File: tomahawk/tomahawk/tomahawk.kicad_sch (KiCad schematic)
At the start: 79 parts, among them SW1 SW_Push, SW10 SW_Push, SW11 SW_Push, SW12 SW_Push, SW13 SW_Push, SW14 SW_Push, SW15 SW_Push, SW16 SW_Push, SW17 SW_Push, SW18 SW_Push, SW19 SW_Push, SW2 SW_Push, SW20 SW_Push, SW21 SW_Push, SW22 SW_Push, SW23 SW_Push, SW24 SW_Push, SW25 SW_Push, SW26 SW_Push, SW27 SW_Push, SW28 SW_Push, SW29 SW_Push, SW3 SW_Push, SW30 SW_Push, SW31 SW_Push, SW32 SW_Push, SW33 SW_Push, SW34 SW_Push, SW35 SW_Push, SW36 SW_Push, SW37 SW_Push, SW38 SW_Push, SW39 SW_Push, SW4 SW_Push, SW5 SW_Push, SW6 SW_Push, SW7 SW_Push, SW8 SW_Push, SW9 SW_Push

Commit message: updated footprints and pcb
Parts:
- SW1, SW10, SW11, SW12, SW13, SW14, SW15, SW16, SW17, SW18, SW19, SW2, SW20, SW21, SW22, SW23, SW24, SW25, SW26, SW27, SW28, SW29, SW3, SW30, SW31, SW32, SW33, SW34, SW35, SW36, SW37, SW38, SW39, SW4, SW5, SW6, SW7, SW8, SW9: footprint Keyswitches:Kailh_socket_PG1350 -> Foostan:keyswitch_choc12_hotswap_1u
- U1: footprint ProMicro_RP2040:pro_micro_rp2040 -> ProMicro RP2040:pro_micro_rp2040
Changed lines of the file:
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@@
 			)
 		)
-		(property "Footprint" "Keyswitches:Kailh_socket_PG1350"
+		(property "Footprint" "Foostan:keyswitch_choc12_hotswap_1u"
 			(at 43.18 90.17 0)
 			(effects
@@
 			)
 		)
-		(property "Footprint" "Keyswitches:Kailh_socket_PG1350"
+		(property "Footprint" "Foostan:keyswitch_choc12_hotswap_1u"
 			(at 43.18 33.02 0)
 			(effects
@@
 			)
 		)
-		(property "Footprint" "Keyswitches:Kailh_socket_PG1350"
+		(property "Footprint" "Foostan:keyswitch_choc12_hotswap_1u"
 			(at 119.38 90.17 0)
 			(effects
@@
 			)
 		)
-		(property "Footprint" "Keyswitches:Kailh_socket_PG1350"
+		(property "Footprint" "Foostan:keyswitch_choc12_hotswap_1u"
 			(at 138.43 33.02 0)
 			(effects
@@
 			)
 		)
-		(property "Footprint" "Keyswitches:Kailh_socket_PG1350"
+		(property "Footprint" "Foostan:keyswitch_choc12_hotswap_1u"
 			(at 119.38 147.32 0)
 			(effects
@@
 			)
 		)
-		(property "Footprint" "Keyswitches:Kailh_socket_PG1350"
+		(property "Footprint" "Foostan:keyswitch_choc12_hotswap_1u"
 			(at 43.18 52.07 0)
 			(effects
@@
 			)
 		)
-		(property "Footprint" "Keyswitches:Kailh_socket_PG1350"
+		(property "Footprint" "Foostan:keyswitch_choc12_hotswap_1u"
 			(at 81.28 147.32 0)
 			(effects
@@
 			)
 		)
-		(property "Footprint" "Keyswitches:Kailh_socket_PG1350"
+		(property "Footprint" "Foostan:keyswitch_choc12_hotswap_1u"
 			(at 81.28 71.12 0)
 			(effects
@@
 			)
 		)
-		(property "Footprint" "ProMicro_RP2040:pro_micro_rp2040"
+		(property "Footprint" "ProMicro RP2040:pro_micro_rp2040"
 			(at 198.12 31.75 0)
 			(effects
@@
 			)
 		)
-		(property "Footprint" "Keyswitches:Kailh_socket_PG1350"
+		(property "Footprint" "Foostan:keyswitch_choc12_hotswap_1u"
 			(at 100.33 128.27 0)
 			(effects
@@
 			)
 		)
-		(property "Footprint" "Keyswitches:Kailh_socket_PG1350"
+		(property "Footprint" "Foostan:keyswitch_choc12_hotswap_1u"
 			(at 138.43 109.22 0)
 			(effects
@@
 			)
 		)
-		(property "Footprint" "Keyswitches:Kailh_socket_PG1350"
+		(property "Footprint" "Foostan:keyswitch_choc12_hotswap_1u"
 			(at 100.33 71.12 0)
 			(effects
@@
 			)
 		)
-		(property "Footprint" "Keyswitches:Kailh_socket_PG1350"
+		(property "Footprint" "Foostan:keyswitch_choc12_hotswap_1u"
 			(at 138.43 90.17 0)
 			(effects
@@
 			)
 		)
-		(property "Footprint" "Keyswitches:Kailh_socket_PG1350"
+		(property "Footprint" "Foostan:keyswitch_choc12_hotswap_1u"
 			(at 62.23 52.07 0)
 			(effects
@@
 			)
 		)
-		(property "Footprint" "Keyswitches:Kailh_socket_PG1350"
+		(property "Footprint" "Foostan:keyswitch_choc12_hotswap_1u"
 			(at 62.23 109.22 0)
 			(effects
@@
 			)
 		)
-		(property "Footprint" "Keyswitches:Kailh_socket_PG1350"
+		(property "Footprint" "Foostan:keyswitch_choc12_hotswap_1u"
 			(at 43.18 71.12 0)
 			(effects
@@
 			)
 		)
-		(property "Footprint" "Keyswitches:Kailh_socket_PG1350"
+		(property "Footprint" "Foostan:keyswitch_choc12_hotswap_1u"
 			(at 100.33 90.17 0)
 			(effects
@@
 			)
 		)
-		(property "Footprint" "Keyswitches:Kailh_socket_PG1350"
+		(property "Footprint" "Foostan:keyswitch_choc12_hotswap_1u"
 			(at 119.38 71.12 0)
 			(effects
@@
 			)
 		)
-		(property "Footprint" "Keyswitches:Kailh_socket_PG1350"
+		(property "Footprint" "Foostan:keyswitch_choc12_hotswap_1u"
 			(at 119.38 52.07 0)
 			(effects
@@
 			)
 		)
-		(property "Footprint" "Keyswitches:Kailh_socket_PG1350"
+		(property "Footprint" "Foostan:keyswitch_choc12_hotswap_1u"
 			(at 119.38 33.02 0)
 			(effects
@@
 			)
 		)
-		(property "Footprint" "Keyswitches:Kailh_socket_PG1350"
+		(property "Footprint" "Foostan:keyswitch_choc12_hotswap_1u"
 			(at 81.28 33.02 0)
 			(effects
@@
 			)
 		)
-		(property "Footprint" "Keyswitches:Kailh_socket_PG1350"
+		(property "Footprint" "Foostan:keyswitch_choc12_hotswap_1u"
 			(at 100.33 166.37 0)
 			(effects
@@
 			)
 		)
-		(property "Footprint" "Keyswitches:Kailh_socket_PG1350"
+		(property "Footprint" "Foostan:keyswitch_choc12_hotswap_1u"
 			(at 138.43 52.07 0)
 			(effects
@@
 			)
 		)
-		(property "Footprint" "Keyswitches:Kailh_socket_PG1350"
+		(property "Footprint" "Foostan:keyswitch_choc12_hotswap_1u"
 			(at 100.33 52.07 0)
 			(effects
@@
 			)
 		)
-		(property "Footprint" "Keyswitches:Kailh_socket_PG1350"
+		(property "Footprint" "Foostan:keyswitch_choc12_hotswap_1u"
 			(at 81.28 128.27 0)
 			(effects
@@
 			)
 		)
-		(property "Footprint" "Keyswitches:Kailh_socket_PG1350"
+		(property "Footprint" "Foostan:keyswitch_choc12_hotswap_1u"
 			(at 62.23 71.12 0)
 			(effects
@@
 			)
 		)
-		(property "Footprint" "Keyswitches:Kailh_socket_PG1350"
+		(property "Footprint" "Foostan:keyswitch_choc12_hotswap_1u"
 			(at 81.28 166.37 0)
 			(effects
@@
 			)
 		)
-		(property "Footprint" "Keyswitches:Kailh_socket_PG1350"
+		(property "Footprint" "Foostan:keyswitch_choc12_hotswap_1u"
 			(at 100.33 109.22 0)
 			(effects
@@
 			)
 		)
-		(property "Footprint" "Keyswitches:Kailh_socket_PG1350"
+		(property "Footprint" "Foostan:keyswitch_choc12_hotswap_1u"
 			(at 81.28 109.22 0)
 			(effects
@@
 			)
 		)
-		(property "Footprint" "Keyswitches:Kailh_socket_PG1350"
+		(property "Footprint" "Foostan:keyswitch_choc12_hotswap_1u"
 			(at 119.38 109.22 0)
 			(effects
@@
 			)
 		)
-		(property "Footprint" "Keyswitches:Kailh_socket_PG1350"
+		(property "Footprint" "Foostan:keyswitch_choc12_hotswap_1u"
 			(at 138.43 71.12 0)
 			(effects
@@
 			)
 		)
-		(property "Footprint" "Keyswitches:Kailh_socket_PG1350"
+		(property "Footprint" "Foostan:keyswitch_choc12_hotswap_1u"
 			(at 62.23 33.02 0)
 			(effects
@@
 			)
 		)
-		(property "Footprint" "Keyswitches:Kailh_socket_PG1350"
+		(property "Footprint" "Foostan:keyswitch_choc12_hotswap_1u"
 			(at 100.33 33.02 0)
 			(effects
@@
 			)
 		)
-		(property "Footprint" "Keyswitches:Kailh_socket_PG1350"
+		(property "Footprint" "Foostan:keyswitch_choc12_hotswap_1u"
 			(at 43.18 109.22 0)
 			(effects
@@
 			)
 		)
-		(property "Footprint" "Keyswitches:Kailh_socket_PG1350"
+		(property "Footprint" "Foostan:keyswitch_choc12_hotswap_1u"
 			(at 62.23 90.17 0)
 			(effects
@@
 			)
 		)
-		(property "Footprint" "Keyswitches:Kailh_socket_PG1350"
+		(property "Footprint" "Foostan:keyswitch_choc12_hotswap_1u"
 			(at 81.28 90.17 0)
 			(effects
@@
 			)
 		)
-		(property "Footprint" "Keyswitches:Kailh_socket_PG1350"
+		(property "Footprint" "Foostan:keyswitch_choc12_hotswap_1u"
 			(at 119.38 128.27 0)
 			(effects
@@
 			)
 		)
-		(property "Footprint" "Keyswitches:Kailh_socket_PG1350"
+		(property "Footprint" "Foostan:keyswitch_choc12_hotswap_1u"
 			(at 100.33 147.32 0)
 			(effects
@@
 			)
 		)
-		(property "Footprint" "Keyswitches:Kailh_socket_PG1350"
+		(property "Footprint" "Foostan:keyswitch_choc12_hotswap_1u"
 			(at 119.38 166.37 0)
 			(effects
@@
 			)
 		)
-		(property "Footprint" "Keyswitches:Kailh_socket_PG1350"
+		(property "Footprint" "Foostan:keyswitch_choc12_hotswap_1u"
 			(at 81.28 52.07 0)
 			(effects

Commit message: updated layout and pcb
- still need to work on the thumb cluster
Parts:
- SW1, SW10, SW11, SW12, SW13, SW14, SW15, SW16, SW17, SW18, SW19, SW2, SW20, SW21, SW22, SW23, SW24, SW25, SW26, SW27, SW28, SW29, SW3, SW30, SW31, SW32, SW33, SW34, SW35, SW36, SW37, SW38, SW39, SW4, SW5, SW6, SW7, SW8, SW9: footprint Foostan:keyswitch_choc12_hotswap_1u -> Scotto Hotswap:Hotswap_Choc_V1V2_1.00u
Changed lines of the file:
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@@
 			)
 		)
-		(property "Footprint" "Foostan:keyswitch_choc12_hotswap_1u"
+		(property "Footprint" "Scotto Hotswap:Hotswap_Choc_V1V2_1.00u"
 			(at 43.18 90.17 0)
 			(effects
@@
 			)
 		)
-		(property "Footprint" "Foostan:keyswitch_choc12_hotswap_1u"
+		(property "Footprint" "Scotto Hotswap:Hotswap_Choc_V1V2_1.00u"
 			(at 43.18 33.02 0)
 			(effects
@@
 			)
 		)
-		(property "Footprint" "Foostan:keyswitch_choc12_hotswap_1u"
+		(property "Footprint" "Scotto Hotswap:Hotswap_Choc_V1V2_1.00u"
 			(at 119.38 90.17 0)
 			(effects
@@
 			)
 		)
-		(property "Footprint" "Foostan:keyswitch_choc12_hotswap_1u"
+		(property "Footprint" "Scotto Hotswap:Hotswap_Choc_V1V2_1.00u"
 			(at 138.43 33.02 0)
 			(effects
@@
 			)
 		)
-		(property "Footprint" "Foostan:keyswitch_choc12_hotswap_1u"
+		(property "Footprint" "Scotto Hotswap:Hotswap_Choc_V1V2_1.00u"
 			(at 119.38 147.32 0)
 			(effects
@@
 			)
 		)
-		(property "Footprint" "Foostan:keyswitch_choc12_hotswap_1u"
+		(property "Footprint" "Scotto Hotswap:Hotswap_Choc_V1V2_1.00u"
 			(at 43.18 52.07 0)
 			(effects
@@
 			)
 		)
-		(property "Footprint" "Foostan:keyswitch_choc12_hotswap_1u"
+		(property "Footprint" "Scotto Hotswap:Hotswap_Choc_V1V2_1.00u"
 			(at 81.28 147.32 0)
 			(effects
@@
 			)
 		)
-		(property "Footprint" "Foostan:keyswitch_choc12_hotswap_1u"
+		(property "Footprint" "Scotto Hotswap:Hotswap_Choc_V1V2_1.00u"
 			(at 81.28 71.12 0)
 			(effects
@@
 			)
 		)
-		(property "Footprint" "Foostan:keyswitch_choc12_hotswap_1u"
+		(property "Footprint" "Scotto Hotswap:Hotswap_Choc_V1V2_1.00u"
 			(at 100.33 128.27 0)
 			(effects
@@
 			)
 		)
-		(property "Footprint" "Foostan:keyswitch_choc12_hotswap_1u"
+		(property "Footprint" "Scotto Hotswap:Hotswap_Choc_V1V2_1.00u"
 			(at 138.43 109.22 0)
 			(effects
@@
 			)
 		)
-		(property "Footprint" "Foostan:keyswitch_choc12_hotswap_1u"
+		(property "Footprint" "Scotto Hotswap:Hotswap_Choc_V1V2_1.00u"
 			(at 100.33 71.12 0)
 			(effects
@@
 			)
 		)
-		(property "Footprint" "Foostan:keyswitch_choc12_hotswap_1u"
+		(property "Footprint" "Scotto Hotswap:Hotswap_Choc_V1V2_1.00u"
 			(at 138.43 90.17 0)
 			(effects
@@
 			)
 		)
-		(property "Footprint" "Foostan:keyswitch_choc12_hotswap_1u"
+		(property "Footprint" "Scotto Hotswap:Hotswap_Choc_V1V2_1.00u"
 			(at 62.23 52.07 0)
 			(effects
@@
 			)
 		)
-		(property "Footprint" "Foostan:keyswitch_choc12_hotswap_1u"
+		(property "Footprint" "Scotto Hotswap:Hotswap_Choc_V1V2_1.00u"
 			(at 62.23 109.22 0)
 			(effects
@@
 			)
 		)
-		(property "Footprint" "Foostan:keyswitch_choc12_hotswap_1u"
+		(property "Footprint" "Scotto Hotswap:Hotswap_Choc_V1V2_1.00u"
 			(at 43.18 71.12 0)
 			(effects
@@
 			)
 		)
-		(property "Footprint" "Foostan:keyswitch_choc12_hotswap_1u"
+		(property "Footprint" "Scotto Hotswap:Hotswap_Choc_V1V2_1.00u"
 			(at 100.33 90.17 0)
 			(effects
@@
 			)
 		)
-		(property "Footprint" "Foostan:keyswitch_choc12_hotswap_1u"
+		(property "Footprint" "Scotto Hotswap:Hotswap_Choc_V1V2_1.00u"
 			(at 119.38 71.12 0)
 			(effects
@@
 			)
 		)
-		(property "Footprint" "Foostan:keyswitch_choc12_hotswap_1u"
+		(property "Footprint" "Scotto Hotswap:Hotswap_Choc_V1V2_1.00u"
 			(at 119.38 52.07 0)
 			(effects
@@
 			)
 		)
-		(property "Footprint" "Foostan:keyswitch_choc12_hotswap_1u"
+		(property "Footprint" "Scotto Hotswap:Hotswap_Choc_V1V2_1.00u"
 			(at 119.38 33.02 0)
 			(effects
@@
 			)
 		)
-		(property "Footprint" "Foostan:keyswitch_choc12_hotswap_1u"
+		(property "Footprint" "Scotto Hotswap:Hotswap_Choc_V1V2_1.00u"
 			(at 81.28 33.02 0)
 			(effects
@@
 			)
 		)
-		(property "Footprint" "Foostan:keyswitch_choc12_hotswap_1u"
+		(property "Footprint" "Scotto Hotswap:Hotswap_Choc_V1V2_1.00u"
 			(at 100.33 166.37 0)
 			(effects
@@
 			)
 		)
-		(property "Footprint" "Foostan:keyswitch_choc12_hotswap_1u"
+		(property "Footprint" "Scotto Hotswap:Hotswap_Choc_V1V2_1.00u"
 			(at 138.43 52.07 0)
 			(effects
@@
 			)
 		)
-		(property "Footprint" "Foostan:keyswitch_choc12_hotswap_1u"
+		(property "Footprint" "Scotto Hotswap:Hotswap_Choc_V1V2_1.00u"
 			(at 100.33 52.07 0)
 			(effects
@@
 			)
 		)
-		(property "Footprint" "Foostan:keyswitch_choc12_hotswap_1u"
+		(property "Footprint" "Scotto Hotswap:Hotswap_Choc_V1V2_1.00u"
 			(at 81.28 128.27 0)
 			(effects
@@
 			)
 		)
-		(property "Footprint" "Foostan:keyswitch_choc12_hotswap_1u"
+		(property "Footprint" "Scotto Hotswap:Hotswap_Choc_V1V2_1.00u"
 			(at 62.23 71.12 0)
 			(effects
@@
 			)
 		)
-		(property "Footprint" "Foostan:keyswitch_choc12_hotswap_1u"
+		(property "Footprint" "Scotto Hotswap:Hotswap_Choc_V1V2_1.00u"
 			(at 81.28 166.37 0)
 			(effects
@@
 			)
 		)
-		(property "Footprint" "Foostan:keyswitch_choc12_hotswap_1u"
+		(property "Footprint" "Scotto Hotswap:Hotswap_Choc_V1V2_1.00u"
 			(at 100.33 109.22 0)
 			(effects
@@
 			)
 		)
-		(property "Footprint" "Foostan:keyswitch_choc12_hotswap_1u"
+		(property "Footprint" "Scotto Hotswap:Hotswap_Choc_V1V2_1.00u"
 			(at 81.28 109.22 0)
 			(effects
@@
 			)
 		)
-		(property "Footprint" "Foostan:keyswitch_choc12_hotswap_1u"
+		(property "Footprint" "Scotto Hotswap:Hotswap_Choc_V1V2_1.00u"
 			(at 119.38 109.22 0)
 			(effects
@@
 			)
 		)
-		(property "Footprint" "Foostan:keyswitch_choc12_hotswap_1u"
+		(property "Footprint" "Scotto Hotswap:Hotswap_Choc_V1V2_1.00u"
 			(at 138.43 71.12 0)
 			(effects
@@
 			)
 		)
-		(property "Footprint" "Foostan:keyswitch_choc12_hotswap_1u"
+		(property "Footprint" "Scotto Hotswap:Hotswap_Choc_V1V2_1.00u"
 			(at 62.23 33.02 0)
 			(effects
@@
 			)
 		)
-		(property "Footprint" "Foostan:keyswitch_choc12_hotswap_1u"
+		(property "Footprint" "Scotto Hotswap:Hotswap_Choc_V1V2_1.00u"
 			(at 100.33 33.02 0)
 			(effects
@@
 			)
 		)
-		(property "Footprint" "Foostan:keyswitch_choc12_hotswap_1u"
+		(property "Footprint" "Scotto Hotswap:Hotswap_Choc_V1V2_1.00u"
 			(at 43.18 109.22 0)
 			(effects
@@
 			)
 		)
-		(property "Footprint" "Foostan:keyswitch_choc12_hotswap_1u"
+		(property "Footprint" "Scotto Hotswap:Hotswap_Choc_V1V2_1.00u"
 			(at 62.23 90.17 0)
 			(effects
@@
 			)
 		)
-		(property "Footprint" "Foostan:keyswitch_choc12_hotswap_1u"
+		(property "Footprint" "Scotto Hotswap:Hotswap_Choc_V1V2_1.00u"
 			(at 81.28 90.17 0)
 			(effects
@@
 			)
 		)
-		(property "Footprint" "Foostan:keyswitch_choc12_hotswap_1u"
+		(property "Footprint" "Scotto Hotswap:Hotswap_Choc_V1V2_1.00u"
 			(at 119.38 128.27 0)
 			(effects
@@
 			)
 		)
-		(property "Footprint" "Foostan:keyswitch_choc12_hotswap_1u"
+		(property "Footprint" "Scotto Hotswap:Hotswap_Choc_V1V2_1.00u"
 			(at 100.33 147.32 0)
 			(effects
@@
 			)
 		)
-		(property "Footprint" "Foostan:keyswitch_choc12_hotswap_1u"
+		(property "Footprint" "Scotto Hotswap:Hotswap_Choc_V1V2_1.00u"
 			(at 119.38 166.37 0)
 			(effects
@@
 			)
 		)
-		(property "Footprint" "Foostan:keyswitch_choc12_hotswap_1u"
+		(property "Footprint" "Scotto Hotswap:Hotswap_Choc_V1V2_1.00u"
 			(at 81.28 52.07 0)
 			(effects

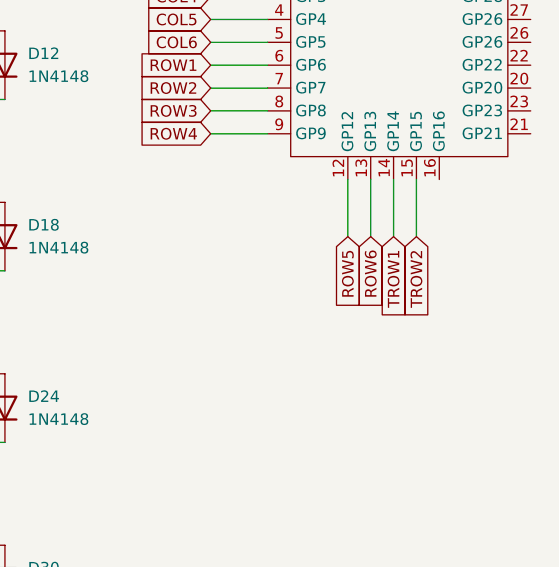
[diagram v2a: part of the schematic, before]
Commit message: rough tracks
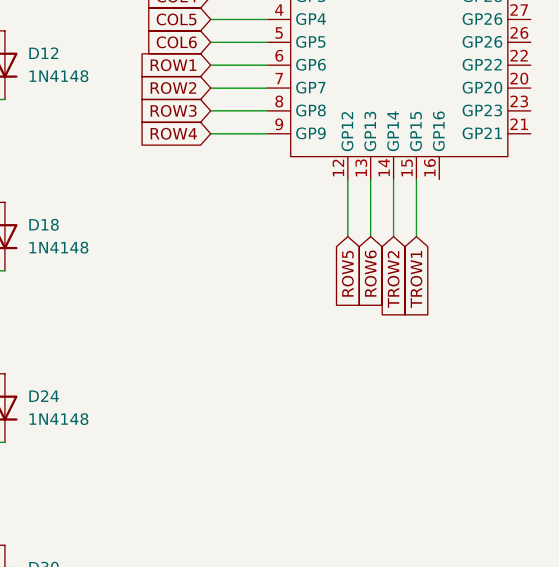
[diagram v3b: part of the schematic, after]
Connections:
- net TROW1: now also U1.15 (GP15); no longer U1.14 (GP14)
- net TROW2: now also U1.14 (GP14); no longer U1.15 (GP15)
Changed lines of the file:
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@@
 	(global_label "TROW2"
 		(shape input)
-		(at 189.23 80.01 270)
+		(at 186.69 80.01 270)
 		(fields_autoplaced yes)
 		(effects
@@
 		)
 		(property "Intersheetrefs" "${INTERSHEET_REFS}"
-			(at 189.23 89.2242 90)
+			(at 186.69 89.2242 90)
 			(effects
 				(font
@@
 	(global_label "TROW1"
 		(shape input)
-		(at 186.69 80.01 270)
+		(at 189.23 80.01 270)
 		(fields_autoplaced yes)
 		(effects
@@
 		)
 		(property "Intersheetrefs" "${INTERSHEET_REFS}"
-			(at 186.69 89.2242 90)
+			(at 189.23 89.2242 90)
 			(effects
 				(font

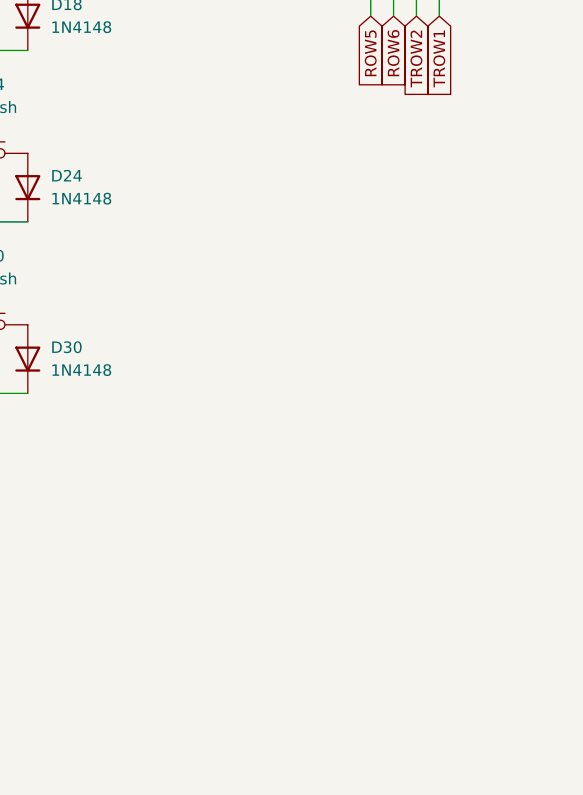
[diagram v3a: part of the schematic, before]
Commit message: wip updated diode positioning, and placed thumb cluster
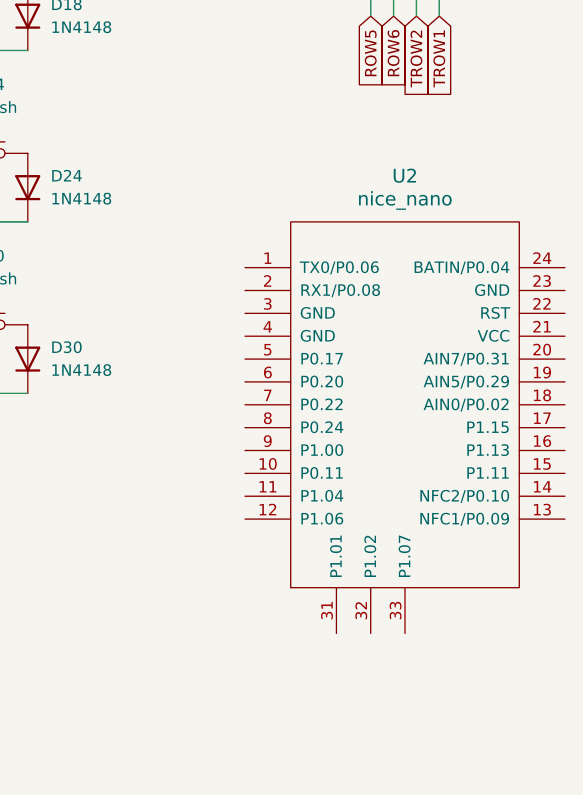
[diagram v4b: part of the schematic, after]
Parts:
- added U2: nice_nano, Scotto MCU:Nice_Nano_V2, symbol nice_nano:nice_nano
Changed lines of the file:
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@@
+	)
+	(symbol
+		(lib_id "nice_nano:nice_nano")
+		(at 185.42 121.92 0)
+		(unit 1)
+		(exclude_from_sim no)
+		(in_bom yes)
+		(on_board yes)
+		(dnp no)
+		(fields_autoplaced yes)
+		(property "Reference" "U2"
+			(at 185.42 97.79 0)
+			(effects
+				(font
+					(size 1.524 1.524)
+				)
+			)
+		)
+		(property "Value" "nice_nano"
+			(at 185.42 100.33 0)
+			(effects
+				(font
+					(size 1.524 1.524)
+				)
+			)
+		)
+		(property "Footprint" "Scotto MCU:Nice_Nano_V2"
+			(at 212.09 185.42 90)
+			(effects
+				(font
+					(size 1.524 1.524)
+				)
+				(hide yes)
+			)
+		)
+		(property "Datasheet" ""
+			(at 212.09 185.42 90)
+			(effects
+				(font
+					(size 1.524 1.524)
+				)
+				(hide yes)
+			)
+		)
+		(property "Description" ""
+			(at 185.42 121.92 0)
+			(effects
+				(font
+					(size 1.27 1.27)
+				)
+				(hide yes)
+			)
+		)
+		(pin "14"
+		)
+		(pin "15"
+		)
+		(pin "18"
+		)
+		(pin "24"
+		)
+		(pin "17"
+		)
+		(pin "16"
+		)
+		(pin "13"
+		)
+		(pin "22"
+		)
+		(pin "10"
+		)
+		(pin "23"
+		)
+		(pin "21"
+		)
+		(pin "6"
+		)
+		(pin "9"
+		)
+		(pin "11"
+		)
+		(pin "19"
+		)
+		(pin "20"
+		)
+		(pin "32"
+		)
+		(pin "12"
+		)
+		(pin "33"
+		)
+		(pin "31"
+		)
+		(pin "7"
+		)
+		(pin "5"
+		)
+		(pin "4"
+		)
+		(pin "3"
+		)
+		(pin "2"
+		)
+		(pin "1"
+		)
+		(pin "8"
+		)
+		(instances
+			(project ""
+				(path "/6c0d08c0-cbd8-49a7-b4b0-a5a869cc48b4"
+					(reference "U2")
+					(unit 1)
+				)
+			)
+		)
 	)
 	(symbol
